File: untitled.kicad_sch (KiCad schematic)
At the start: 36 parts, among them U4 LT1963AEST-3.3#TRPBF, U5 TPS2115ADRBR, U6 TPS5405DR

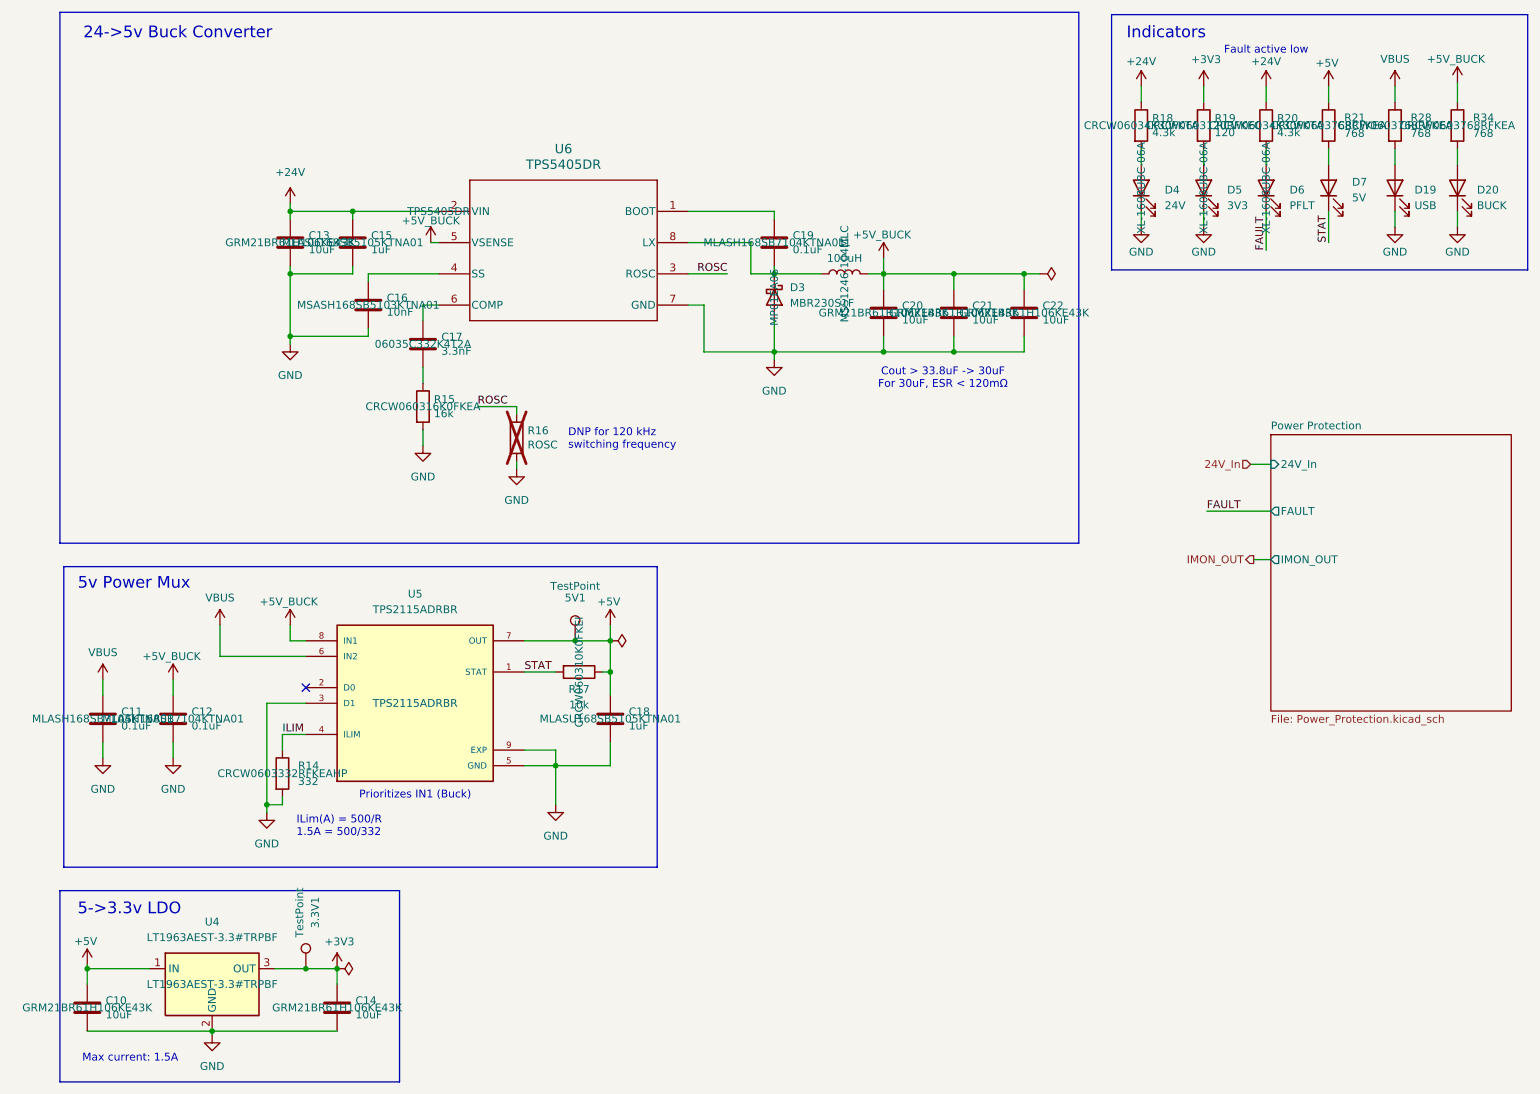
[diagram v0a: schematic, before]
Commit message: power/connectors
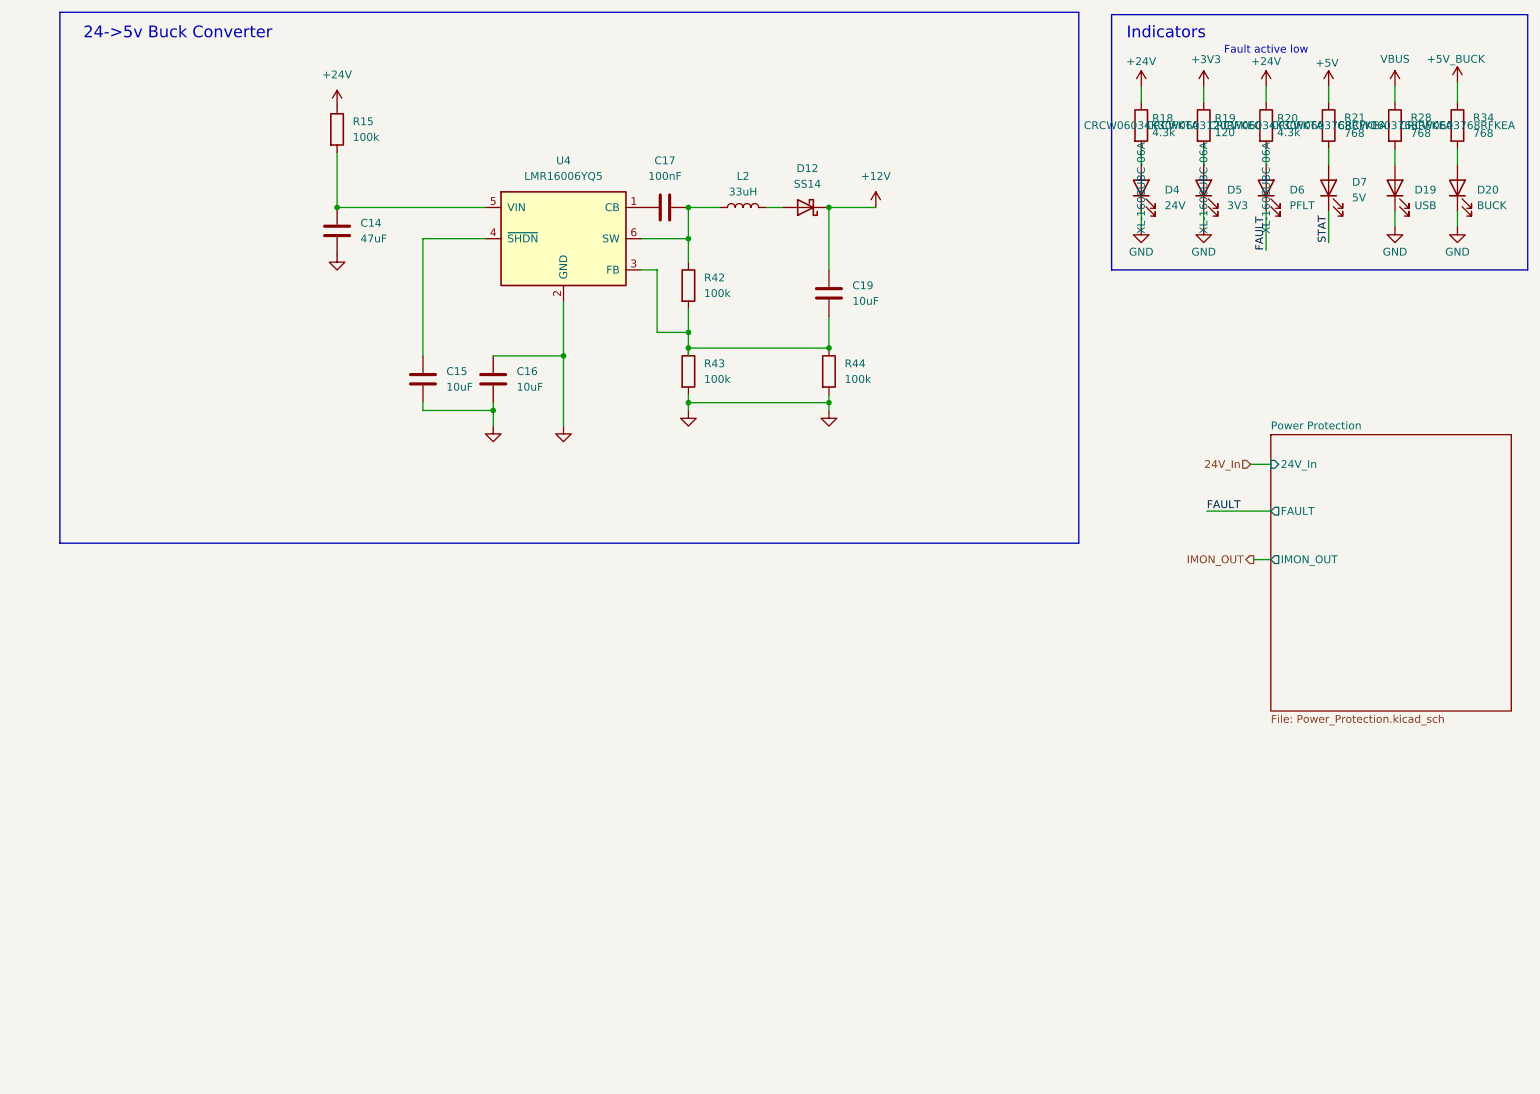
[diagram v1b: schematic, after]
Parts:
- removed 3.3V1, 5V1: TestPoint, TestPoint:TestPoint_Pad_1.0x1.0mm, symbol Connector:TestPoint
- removed C10, C13, C20, C21, C22: 10uF, Capacitor_SMD:C_0805_2012Metric_Pad1.18x1.45mm_HandSolder, symbol Device:C
- removed C11, C12: 0.1uF, Capacitor_SMD:C_0603_1608Metric_Pad1.08x0.95mm_HandSolder, symbol Device:C
- removed C18: 1uF, Capacitor_SMD:C_0603_1608Metric_Pad1.08x0.95mm_HandSolder, symbol Device:C
- removed D3: MBR230S1F, Diode_SMD:D_SOD-123F, symbol Device:D_Schottky
- removed L1: 100uH, Inductor_SMD:L_Coilcraft_MSS1246-XXX, symbol Device:L
- removed R14: 332, Resistor_SMD:R_0603_1608Metric_Pad0.98x0.95mm_HandSolder, symbol Device:R
- removed R16: ROSC, Resistor_SMD:R_0603_1608Metric_Pad0.98x0.95mm_HandSolder, symbol Device:R
- removed R17: 10k, Resistor_SMD:R_0603_1608Metric_Pad0.98x0.95mm_HandSolder, symbol Device:R
- removed U4: LT1963AEST-3.3#TRPBF, Package_TO_SOT_SMD:SOT-223-3_TabPin2, symbol Regulator_Linear:LT1963AxST-3.3
- removed U5: TPS2115ADRBR, TPS2115ABDR:SON65P300X300X100-9N, symbol TPS2115ADBR:TPS2115ADRBR
- removed U6: TPS5405DR, UTSVT_Power:TPS5405DR, symbol UTSVT-Power:TPS5405DR
- added D12: SS14, Diode_SMD:D_SMA, symbol Diode:SS14
- added L2: 33uH, symbol Device:L
- added R42, R43, R44: 100k, symbol Device:R
- added U4: LMR16006YQ5, Package_TO_SOT_SMD:SOT-23-6, symbol Regulator_Switching:LMR16006YQ5
- C14: value 10uF -> 47uF; footprint Capacitor_SMD:C_0805_2012Metric_Pad1.18x1.45mm_HandSolder -> (none); Mouser Part Number GRM21BR61H106KE43K -> (none); P/N GRM21BR61H106KE43K -> (none)
- C15: value 1uF -> 10uF; footprint Capacitor_SMD:C_0603_1608Metric_Pad1.08x0.95mm_HandSolder -> (none); Mouser Part Number MLASU168SB5105KTNA01 -> (none); P/N MLASU168SB5105KTNA01 -> (none)
- C16: value 10nF -> 10uF; footprint Capacitor_SMD:C_0603_1608Metric_Pad1.08x0.95mm_HandSolder -> (none); Mouser Part Number MSASH168SB5103KTNA01 -> (none); P/N MSASH168SB5103KTNA01 -> (none)
- C17: value 3.3nF -> 100nF; footprint Capacitor_SMD:C_0603_1608Metric_Pad1.08x0.95mm_HandSolder -> (none); Mouser Part Number 06035C332K4T2A -> (none); P/N 06035C332K4T2A -> (none)
- C19: value 0.1uF -> 10uF; footprint Capacitor_SMD:C_0603_1608Metric_Pad1.08x0.95mm_HandSolder -> (none); Mouser Part Number MLASH168SB7104KTNA01 -> (none); P/N MLASH168SB7104KTNA01 -> (none)
- R15: value 16k -> 100k; footprint Resistor_SMD:R_0603_1608Metric_Pad0.98x0.95mm_HandSolder -> (none); Mouser Part Number CRCW060316K0FKEA -> (none); P/N CRCW060316K0FKTA -> (none)
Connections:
- net +24V: now also R15.1; no longer C15.1
- net +3V3: no longer C14.1
- net GND: now also C16.1, R43.2, R44.2, U4.2 (GND); no longer R15.2
- net +12V: now reaches C19.1
- net +12V: now also D12.1 (K)
- net at C17.1: now also U4.1 (CB)
- net at C19.2: now also R42.2, R43.1, R44.1, U4.3 (FB)
- net at C17.2: now also L2.1, R42.1, U4.6 (SW); no longer R15.1
- new net: C14.1, R15.2, U4.5 (VIN)
- new net: C15.1, U4.4 (~{SHDN})
- new net: D12.2 (A), L2.2
- no-connect marks 1 -> 0
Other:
- note removed: "5->3.3v LDO"
- note removed: "5v Power Mux"
- note removed: "Cout > 33.8uF -> 30uF For 30uF, ESR < 120mΩ"
- note removed: "DNP for 120 kHz switching frequency"
- note removed: "ILim(A) = 500/R 1.5A = 500/332"
- note removed: "Max current: 1.5A"
- note removed: "Prioritizes IN1 (Buck)"
